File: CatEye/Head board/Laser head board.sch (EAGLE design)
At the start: 17 parts, among them X1 DVI-D-R, X2 SMA-R

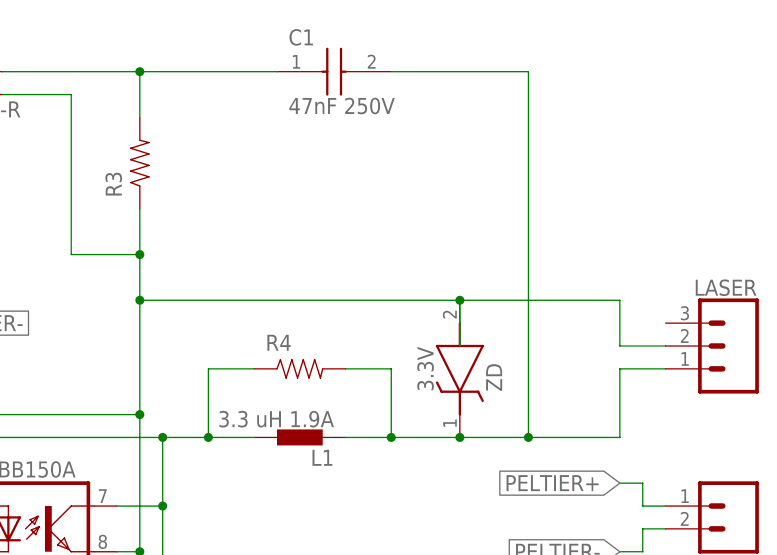
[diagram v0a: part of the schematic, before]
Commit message: Updated EAGLE files
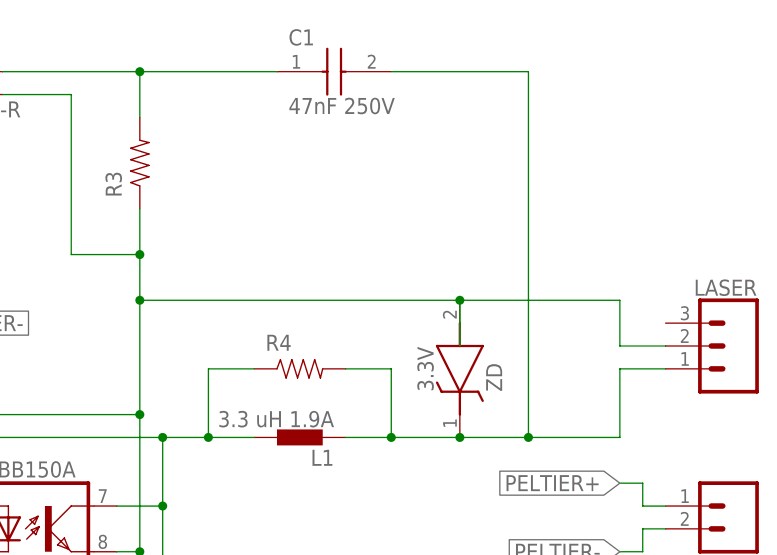
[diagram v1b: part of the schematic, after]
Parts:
- C1: device OCR:C3216X7R2E473K160AA -> headboard:OCR_C3216X7R2E473K160AA
- L1: device OCR:SLF7032T -> headboard:OCR_SLF7032T
- LASER: device OCR:CONN_03 -> headboard:OCR_CONN_03
- LD1: device OCR:WP130WCP/2EGW -> headboard:OCR_WP130WCP/2EGW
- PBB150: device OCR:PBB150 -> headboard:OCR_PBB150
- PIEZO, TEC, THERM: device OCR:CONN_02 -> headboard:OCR_CONN_02
- R1, R2, R3, R4, R5, R6: device OCR:RESISTOR -> headboard:OCR_RESISTOR
- X1: device OCR:DVI-D-R_74320 -> headboard:OCR_DVI-D-R_74320
- X2: device OCR:SMA-R/A -> headboard:OCR_SMA-R/A
- ZD: device OCR:MMSZ3V3T1G -> headboard:OCR_MMSZ3V3T1G
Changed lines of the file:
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@@
 <?xml version="1.0" encoding="utf-8"?>
 <!DOCTYPE eagle SYSTEM "eagle.dtd">
-<eagle version="9.3.0">
+<eagle version="9.6.2">
 <drawing>
 <settings>
@@
 </classes>
 <parts>
-<part name="X2" library="OCR" library_urn="urn:adsk.eagle:library:8062975" deviceset="SMA-R/A" device="" package3d_urn="urn:adsk.eagle:package:8063023/3" value="SMA-R"/>
-<part name="TEC" library="OCR" library_urn="urn:adsk.eagle:library:8062975" deviceset="CONN_02" device="" package3d_urn="urn:adsk.eagle:package:8113090/4"/>
-<part name="PIEZO" library="OCR" library_urn="urn:adsk.eagle:library:8062975" deviceset="CONN_02" device="" package3d_urn="urn:adsk.eagle:package:8113090/4"/>
-<part name="THERM" library="OCR" library_urn="urn:adsk.eagle:library:8062975" deviceset="CONN_02" device="" package3d_urn="urn:adsk.eagle:package:8113090/4"/>
-<part name="LASER" library="OCR" library_urn="urn:adsk.eagle:library:8062975" deviceset="CONN_03" device="" package3d_urn="urn:adsk.eagle:package:8116905/3"/>
-<part name="L1" library="OCR" library_urn="urn:adsk.eagle:library:8062975" deviceset="SLF7032T" device="" package3d_urn="urn:adsk.eagle:package:8063020/4" value="3.3 uH 1.9A"/>
-<part name="R3" library="OCR" library_urn="urn:adsk.eagle:library:8062975" deviceset="RESISTOR" device="" package3d_urn="urn:adsk.eagle:package:8116984/2" value="10k"/>
-<part name="R1" library="OCR" library_urn="urn:adsk.eagle:library:8062975" deviceset="RESISTOR" device="" package3d_urn="urn:adsk.eagle:package:8116984/2" value="390R"/>
-<part name="R6" library="OCR" library_urn="urn:adsk.eagle:library:8062975" deviceset="RESISTOR" device="" package3d_urn="urn:adsk.eagle:package:8116984/2" value="499R"/>
-<part name="R5" library="OCR" library_urn="urn:adsk.eagle:library:8062975" deviceset="RESISTOR" device="" package3d_urn="urn:adsk.eagle:package:8116984/2" value="499R"/>
-<part name="R2" library="OCR" library_urn="urn:adsk.eagle:library:8062975" deviceset="RESISTOR" device="" package3d_urn="urn:adsk.eagle:package:8116984/2" value="4k99"/>
-<part name="R4" library="OCR" library_urn="urn:adsk.eagle:library:8062975" deviceset="RESISTOR" device="" package3d_urn="urn:adsk.eagle:package:8116984/2" value="43R"/>
-<part name="PBB150" library="OCR" library_urn="urn:adsk.eagle:library:8062975" deviceset="PBB150" device="" package3d_urn="urn:adsk.eagle:package:8063021/2"/>
-<part name="X1" library="OCR" library_urn="urn:adsk.eagle:library:8062975" deviceset="DVI-D-R" device="_74320" package3d_urn="urn:adsk.eagle:package:8063018/2" value="DVI-D-R"/>
-<part name="LD1" library="OCR" library_urn="urn:adsk.eagle:library:8062975" deviceset="WP130WCP/2EGW" device="" package3d_urn="urn:adsk.eagle:package:8063024/2"/>
-<part name="ZD" library="OCR" library_urn="urn:adsk.eagle:library:8062975" deviceset="MMSZ3V3T1G" device="" package3d_urn="urn:adsk.eagle:package:8068621/4" value="3.3V"/>
-<part name="C1" library="OCR" library_urn="urn:adsk.eagle:library:8062975" deviceset="C3216X7R2E473K160AA" device="" package3d_urn="urn:adsk.eagle:package:8068922/2" value="47nF 250V"/>
+<part name="X2" library="headboard" library_urn="urn:adsk.eagle:library:49120877" deviceset="OCR_SMA-R/A" device="" package3d_urn="urn:adsk.eagle:package:49120900/1" value="SMA-R"/>
+<part name="TEC" library="headboard" library_urn="urn:adsk.eagle:library:49120877" deviceset="OCR_CONN_02" device="" package3d_urn="urn:adsk.eagle:package:49120902/1"/>
+<part name="PIEZO" library="headboard" library_urn="urn:adsk.eagle:library:49120877" deviceset="OCR_CONN_02" device="" package3d_urn="urn:adsk.eagle:package:49120902/1"/>
+<part name="THERM" library="headboard" library_urn="urn:adsk.eagle:library:49120877" deviceset="OCR_CONN_02" device="" package3d_urn="urn:adsk.eagle:package:49120902/1"/>
+<part name="LASER" library="headboard" library_urn="urn:adsk.eagle:library:49120877" deviceset="OCR_CONN_03" device="" package3d_urn="urn:adsk.eagle:package:49120901/1"/>
+<part name="L1" library="headboard" library_urn="urn:adsk.eagle:library:49120877" deviceset="OCR_SLF7032T" device="" package3d_urn="urn:adsk.eagle:package:49120903/1" value="3.3 uH 1.9A"/>
+<part name="R3" library="headboard" library_urn="urn:adsk.eagle:library:49120877" deviceset="OCR_RESISTOR" device="" package3d_urn="urn:adsk.eagle:package:49120907/1" value="10k"/>
+<part name="R1" library="headboard" library_urn="urn:adsk.eagle:library:49120877" deviceset="OCR_RESISTOR" device="" package3d_urn="urn:adsk.eagle:package:49120907/1" value="390R"/>
+<part name="R6" library="headboard" library_urn="urn:adsk.eagle:library:49120877" deviceset="OCR_RESISTOR" device="" package3d_urn="urn:adsk.eagle:package:49120907/1" value="499R"/>
+<part name="R5" library="headboard" library_urn="urn:adsk.eagle:library:49120877" deviceset="OCR_RESISTOR" device="" package3d_urn="urn:adsk.eagle:package:49120907/1" value="499R"/>
+<part name="R2" library="headboard" library_urn="urn:adsk.eagle:library:49120877" deviceset="OCR_RESISTOR" device="" package3d_urn="urn:adsk.eagle:package:49120907/1" value="4k99"/>
+<part name="R4" library="headboard" library_urn="urn:adsk.eagle:library:49120877" deviceset="OCR_RESISTOR" device="" package3d_urn="urn:adsk.eagle:package:49120907/1" value="43R"/>
+<part name="PBB150" library="headboard" library_urn="urn:adsk.eagle:library:49120877" deviceset="OCR_PBB150" device="" package3d_urn="urn:adsk.eagle:package:49120905/1"/>
+<part name="X1" library="headboard" library_urn="urn:adsk.eagle:library:49120877" deviceset="OCR_DVI-D-R" device="_74320" package3d_urn="urn:adsk.eagle:package:49120904/1" value="DVI-D-R"/>
+<part name="LD1" library="headboard" library_urn="urn:adsk.eagle:library:49120877" deviceset="OCR_WP130WCP/2EGW" device="" package3d_urn="urn:adsk.eagle:package:49120898/1"/>
+<part name="ZD" library="headboard" library_urn="urn:adsk.eagle:library:49120877" deviceset="OCR_MMSZ3V3T1G" device="" package3d_urn="urn:adsk.eagle:package:49120899/1" value="3.3V"/>
+<part name="C1" library="headboard" library_urn="urn:adsk.eagle:library:49120877" deviceset="OCR_C3216X7R2E473K160AA" device="" package3d_urn="urn:adsk.eagle:package:49120906/1" value="47nF 250V"/>
 </parts>
 <sheets>
